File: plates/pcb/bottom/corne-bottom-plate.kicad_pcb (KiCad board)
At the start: 2 copper layers, 133.8 x 91.4 mm, 7 parts

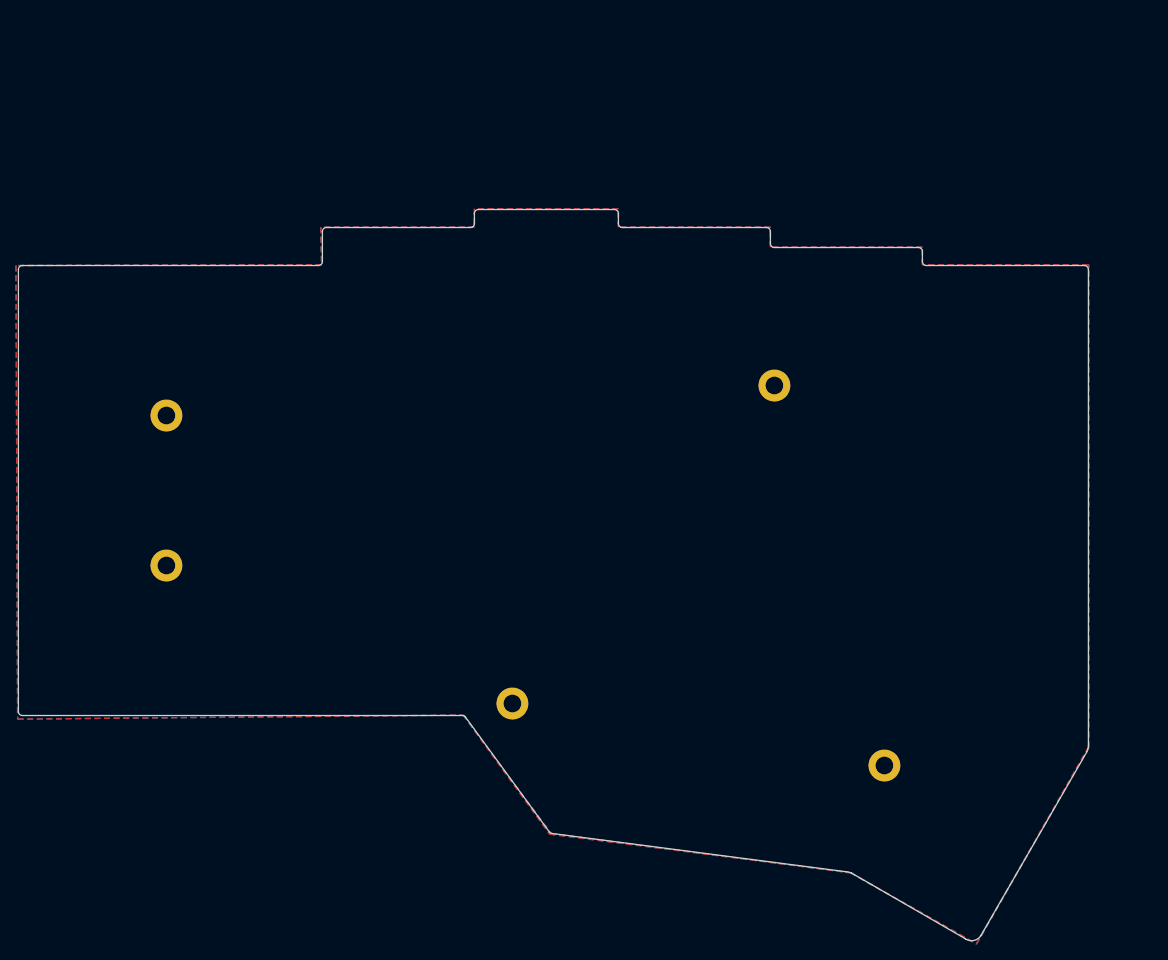
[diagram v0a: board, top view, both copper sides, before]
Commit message: rp2040 v0
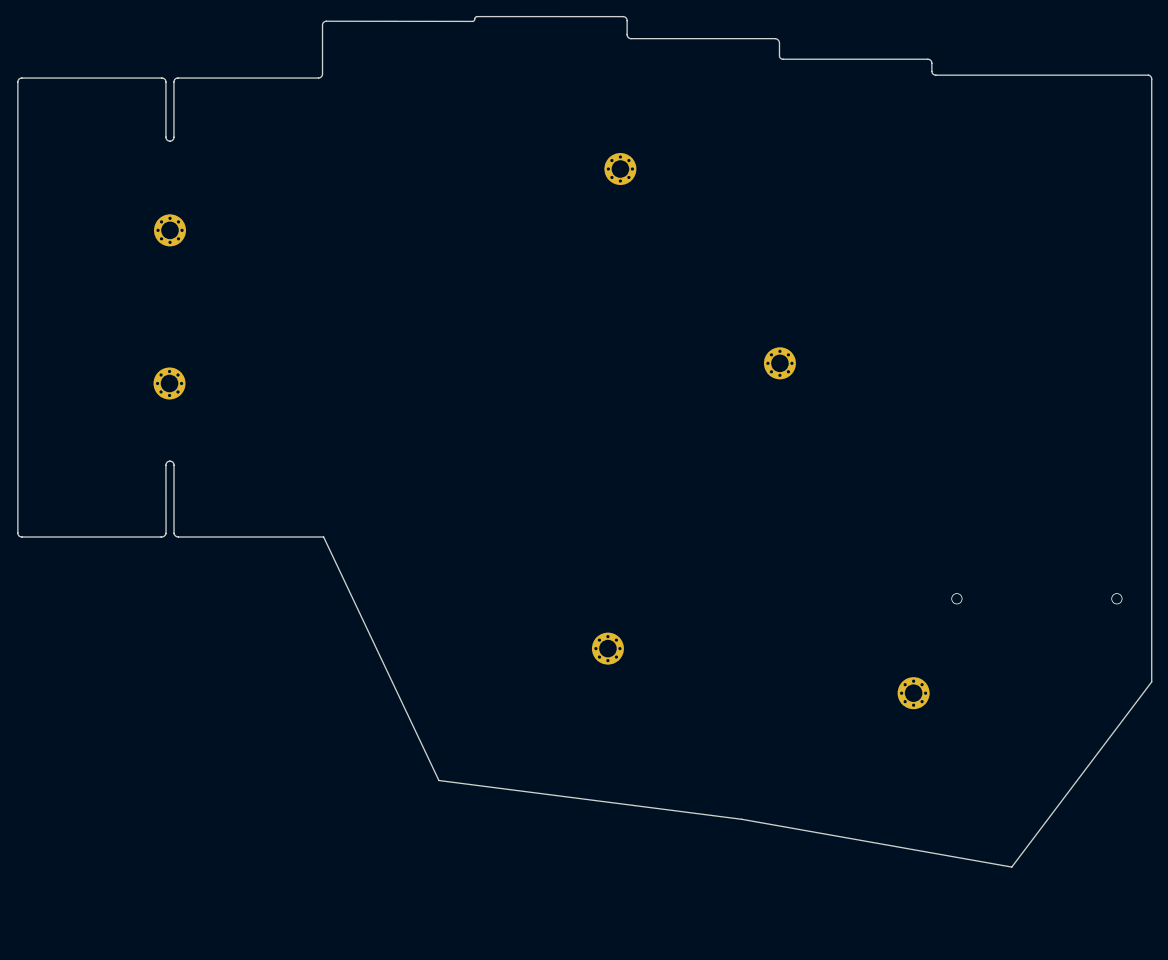
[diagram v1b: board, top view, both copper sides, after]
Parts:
- removed the ? at (79.5, 105.5)
- removed the ? at (79.5, 86.8)
- removed the ? at (155.5, 83.0)
- removed the ? at (122.8, 122.8)
- removed the ? at (169.2, 130.5)
- removed G*** (x2): LOGO, kbd:corne-mask
- added ?: , kbd:M2_HOLE_v3, F.Cu at (80.0, 63.6)
- added ?: , kbd:M2_HOLE_v3, F.Cu at (136.3, 55.9)
- added ?: , kbd:M2_HOLE_v3, F.Cu at (172.9, 121.5)
- added ?: , kbd:M2_HOLE_v3, F.Cu at (79.9, 82.7)
- added ?: , kbd:M2_HOLE_v3, F.Cu at (156.2, 80.2)
- added ?: , kbd:M2_HOLE_v3, F.Cu at (134.7, 115.9)
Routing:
- net (no net): vias 0 -> 2
- removed copper zone on B.Cu, net (none)
- removed copper zone on F.Cu, net (none)
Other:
- board size 133.8 x 91.4 mm -> 141.7 x 106.3 mm
- net class Default removed
